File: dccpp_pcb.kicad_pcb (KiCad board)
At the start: 2 copper layers, 101.6 x 63.5 mm, 71 parts, among them J1 USB_B_Micro, J10 OSTTC022162, J11 OSTTC022162, J12 OSTTC022162, J2 AVR-ISP-6, J3 OSTTC022162, J4 OSTTC022162, J5 OSTTC022162, J6 OSTTC022162, J7 OSTTC022162, J8 OSTTC022162, J9 OSTTC022162, U1 ATmega32U4-AU, U2 74HC04, U3 IFX007T, U4 IFX007T, U5 IFX007T, U6 IFX007T, Y1 16MHz

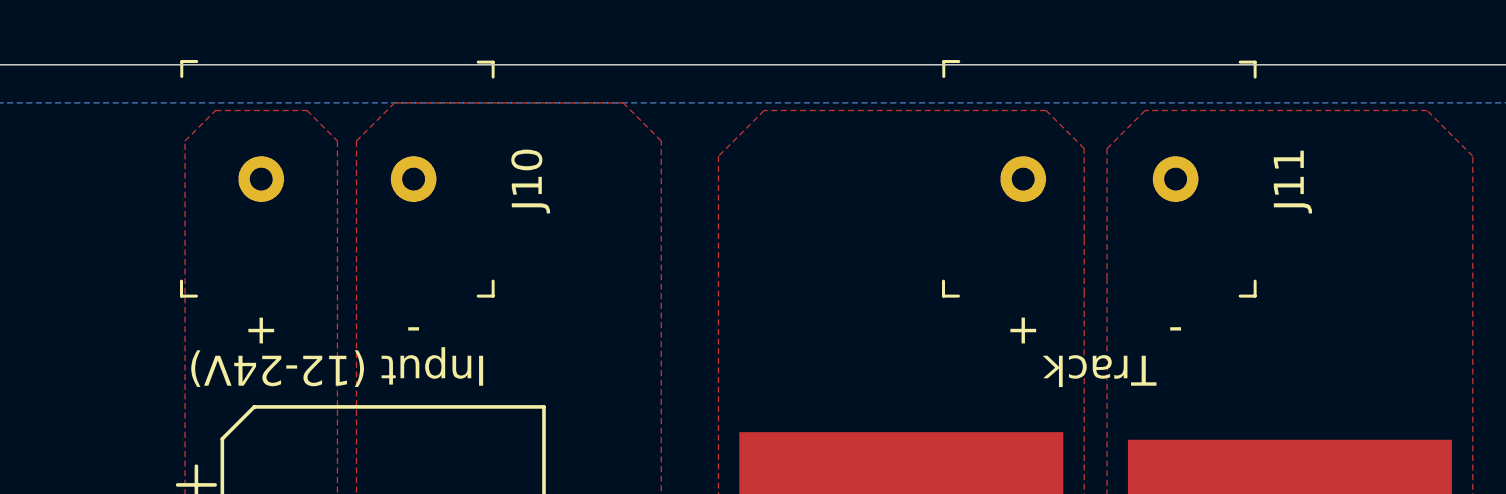
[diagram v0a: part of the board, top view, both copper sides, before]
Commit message: Finished art
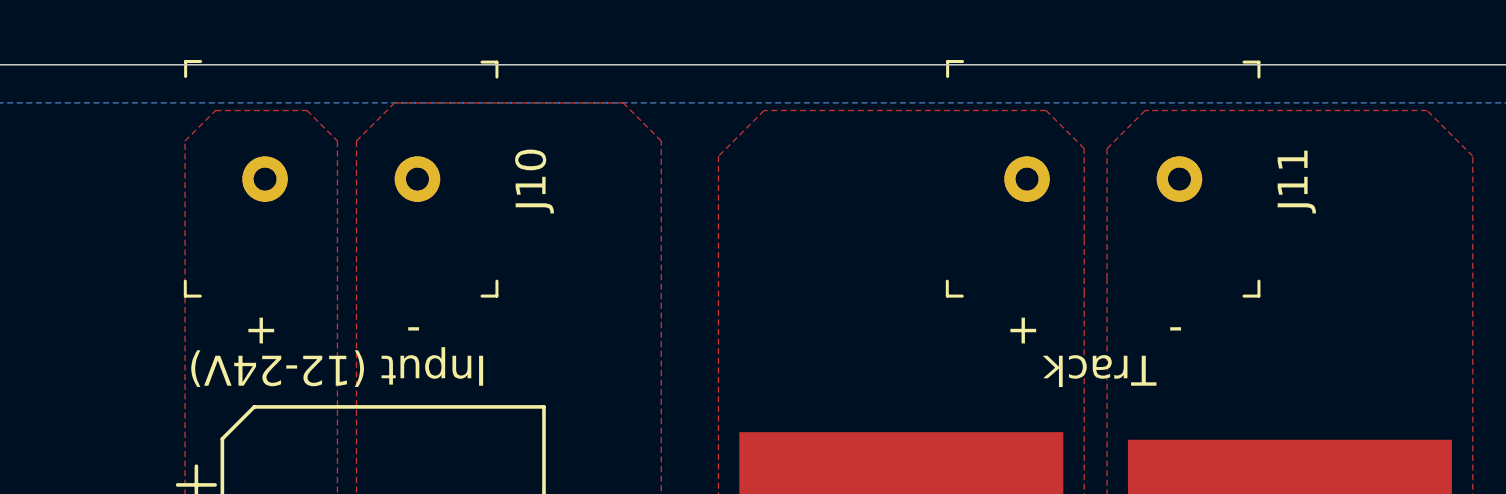
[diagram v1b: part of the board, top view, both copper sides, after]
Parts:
- moved J10 0.13 mm to (91.6, 92.7)
- moved J11 0.13 mm to (117.0, 92.7)
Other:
- board text added: "DCC++"
